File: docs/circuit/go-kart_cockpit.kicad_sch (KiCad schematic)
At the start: 37 parts, among them P1 Power, Q1 TIP120, SW1 SW_MEC_5E, X1 AVR-ISP-10, X10 Bluetooth-Modul, X11 Start/Stop/Rückwärts, X12 Taster rechts (male), X13 Taster links (male), X2 Display (male), X3 5V, X4 GND, X5 SDA, X6 24V Hupe, X7 J5, X8 J3, X9 SCL

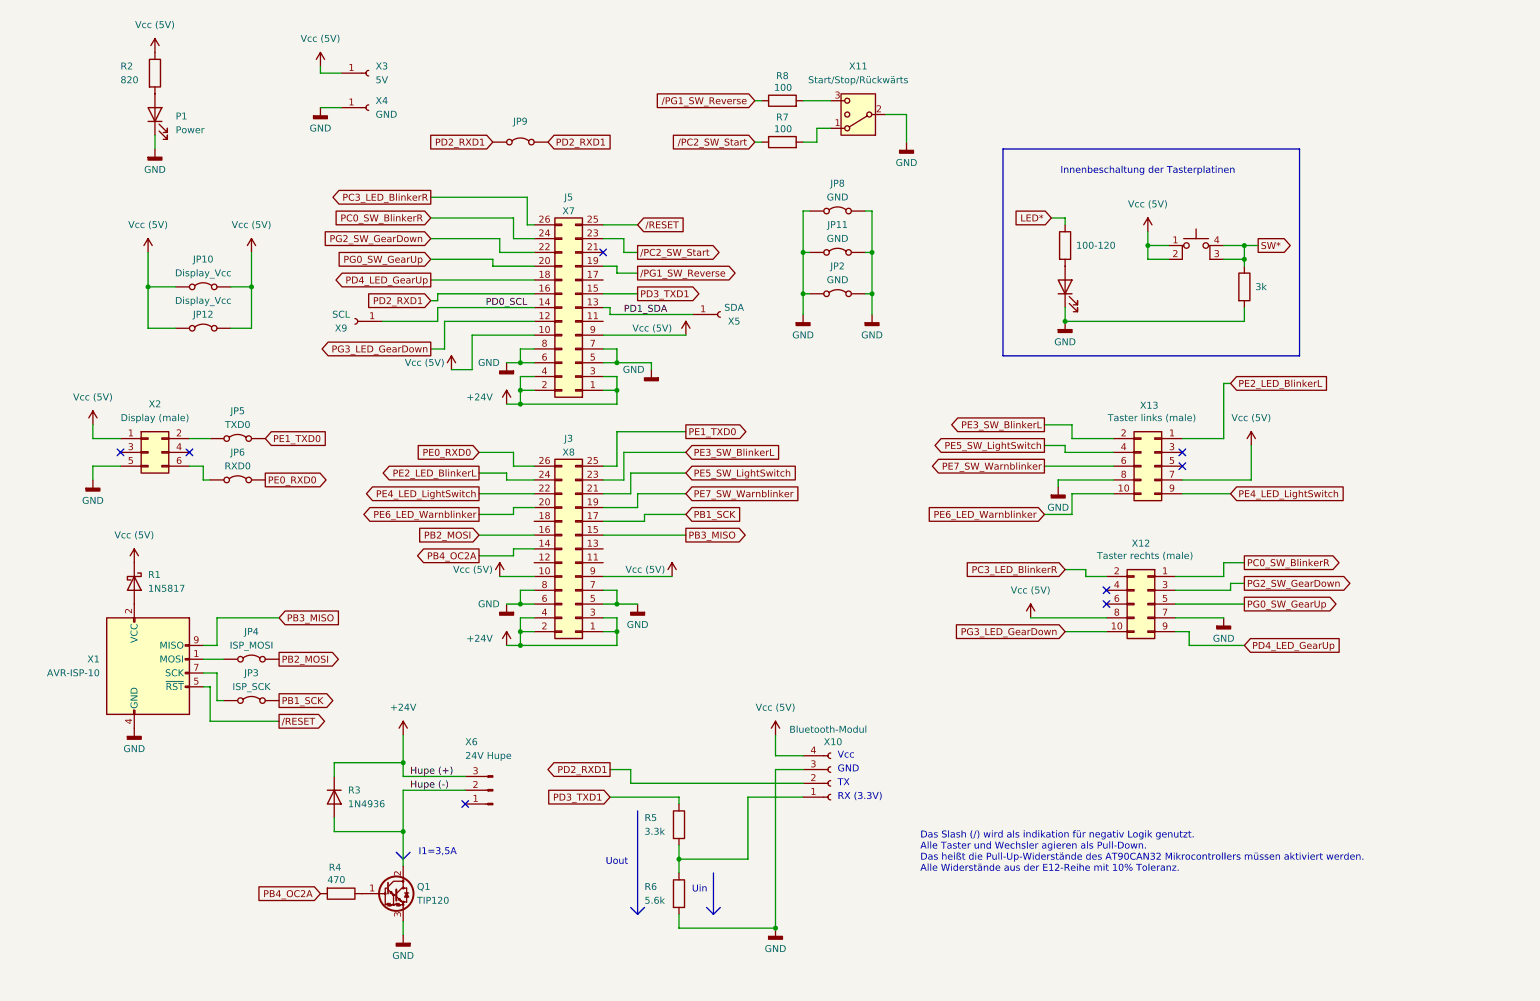
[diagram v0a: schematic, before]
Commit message: feat(circuit): final touches
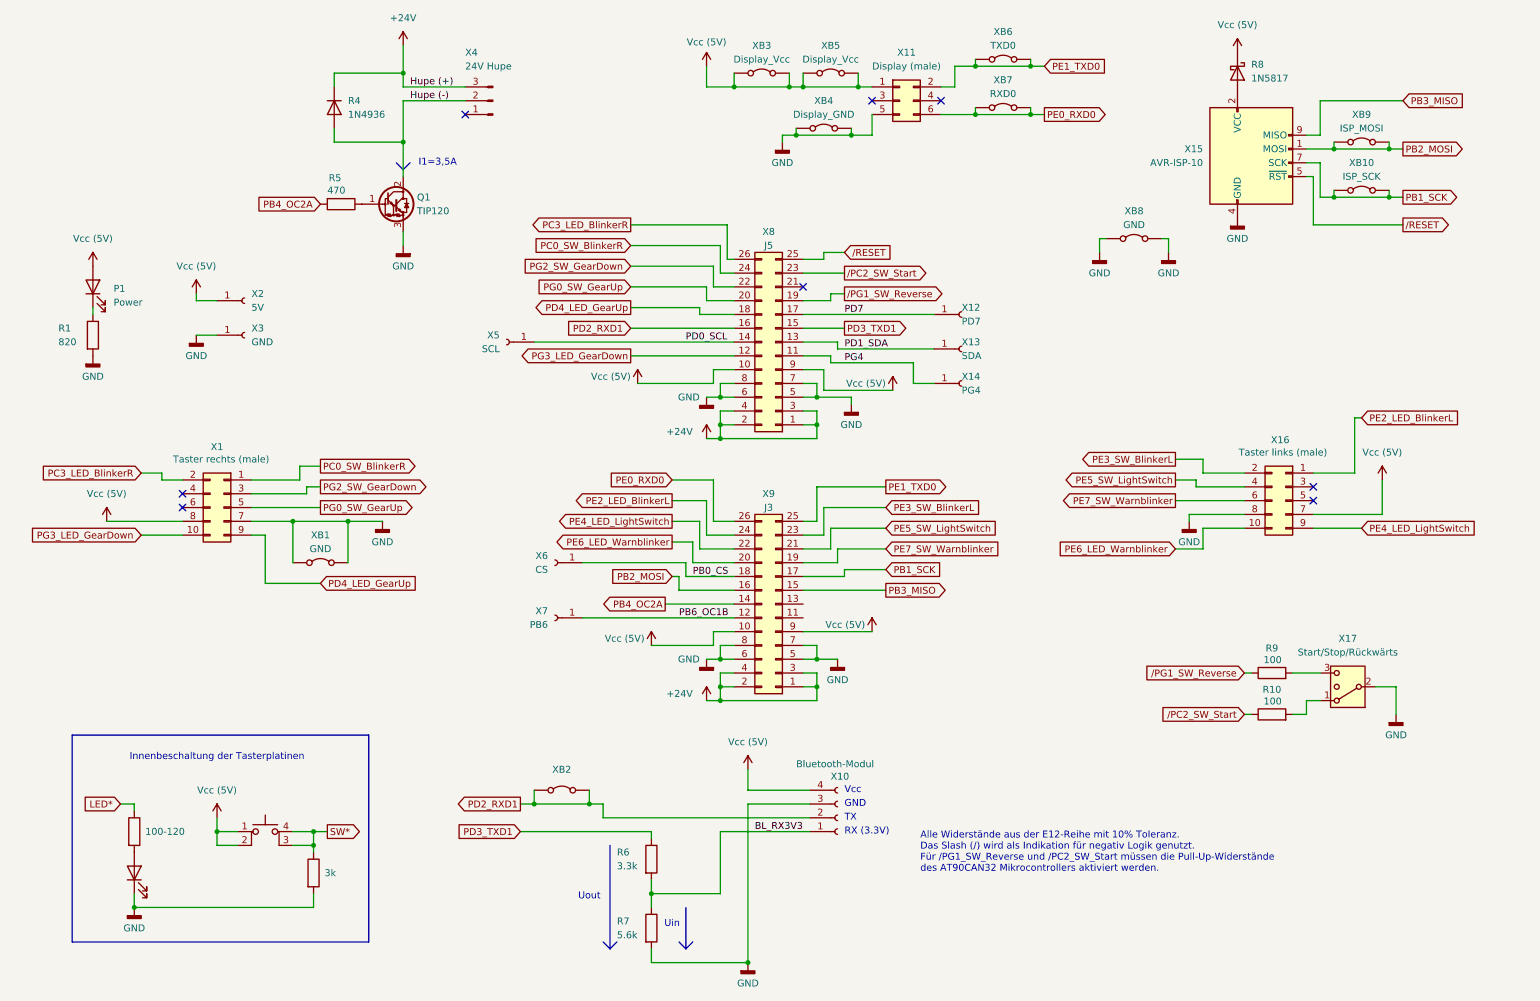
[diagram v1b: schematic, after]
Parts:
- removed JP10: Display_Vcc, Resistor_THT:R_Axial_DIN0207_L6.3mm_D2.5mm_P7.62mm_Horizontal, symbol Jumper:Jumper_2_Bridged
- removed JP12: Display_Vcc, Resistor_THT:R_Axial_DIN0207_L6.3mm_D2.5mm_P15.24mm_Horizontal, symbol Jumper:Jumper_2_Bridged
- removed JP3: ISP_SCK, Resistor_THT:R_Axial_DIN0207_L6.3mm_D2.5mm_P10.16mm_Horizontal, symbol Jumper:Jumper_2_Bridged
- removed JP4: ISP_MOSI, Resistor_THT:R_Axial_DIN0207_L6.3mm_D2.5mm_P15.24mm_Horizontal, symbol Jumper:Jumper_2_Bridged
- removed JP5: TXD0, Resistor_THT:R_Axial_DIN0207_L6.3mm_D2.5mm_P10.16mm_Horizontal, symbol Jumper:Jumper_2_Bridged
- removed JP6: RXD0, Resistor_THT:R_Axial_DIN0207_L6.3mm_D2.5mm_P10.16mm_Horizontal, symbol Jumper:Jumper_2_Bridged
- removed JP9: ~, Resistor_THT:R_Axial_DIN0207_L6.3mm_D2.5mm_P15.24mm_Horizontal, symbol Jumper:Jumper_2_Bridged
- added X12: PD7, Connector_PinSocket_2.54mm:PinSocket_1x01_P2.54mm_Vertical, symbol Connector:Conn_01x01_Socket
- added X14: PG4, Connector_PinSocket_2.54mm:PinSocket_1x01_P2.54mm_Vertical, symbol Connector:Conn_01x01_Socket
- added X6: CS, Connector_PinSocket_2.54mm:PinSocket_1x01_P2.54mm_Vertical, symbol Connector:Conn_01x01_Socket
- added X7: PB6, Connector_PinSocket_2.54mm:PinSocket_1x01_P2.54mm_Vertical, symbol Connector:Conn_01x01_Socket
- added XB10: ISP_SCK, Resistor_THT:R_Axial_DIN0207_L6.3mm_D2.5mm_P10.16mm_Horizontal, symbol Jumper:Jumper_2_Bridged
- added XB2: ~, Resistor_THT:R_Axial_DIN0207_L6.3mm_D2.5mm_P15.24mm_Horizontal, symbol Jumper:Jumper_2_Bridged
- added XB3: Display_Vcc, Resistor_THT:R_Axial_DIN0207_L6.3mm_D2.5mm_P7.62mm_Horizontal, symbol Jumper:Jumper_2_Bridged
- added XB5: Display_Vcc, Resistor_THT:R_Axial_DIN0207_L6.3mm_D2.5mm_P15.24mm_Horizontal, symbol Jumper:Jumper_2_Bridged
- added XB6: TXD0, Resistor_THT:R_Axial_DIN0207_L6.3mm_D2.5mm_P10.16mm_Horizontal, symbol Jumper:Jumper_2_Bridged
- added XB7: RXD0, Resistor_THT:R_Axial_DIN0207_L6.3mm_D2.5mm_P10.16mm_Horizontal, symbol Jumper:Jumper_2_Bridged
- added XB9: ISP_MOSI, Resistor_THT:R_Axial_DIN0207_L6.3mm_D2.5mm_P15.24mm_Horizontal, symbol Jumper:Jumper_2_Bridged
- XB4: renamed from JP8; value GND -> Display_GND
- renumbered R2 to R1, R7 to R10, R9 to R2, R10 to R3, R3 to R4, R4 to R5, R5 to R6, R6 to R7, R1 to R8, R8 to R9, X12 to X1, X2 to X11, X5 to X13, X1 to X15, X13 to X16, X11 to X17, X3 to X2, X4 to X3, X6 to X4, X9 to X5, X7 to X8, X8 to X9, JP11 to XB1, JP2 to XB8
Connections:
- net GND: now also R1.2; no longer P1.1 (K)
- net PB1_SCK: now also X15.7 (SCK), XB10.1 (A), XB10.2 (B)
- net PB2_MOSI: now also X15.1 (MOSI), XB9.1 (A), XB9.2 (B)
- net PD2_RXD1: now also XB2.1 (A), XB2.2 (B)
- net PE0_RXD0: now also X11.6 (Pin_6), XB7.1 (A), XB7.2 (B)
- net PE1_TXD0: now also X11.2 (Pin_2), XB6.1 (A), XB6.2 (B)
- net Vcc (5V): now also P1.2 (A), XB3.1 (A), XB3.2 (B), XB5.1 (A), XB5.2 (B); no longer R1.1
- net BL_RX3V3: now reaches R6.2, R7.1, X10.1 (Pin_1)
- net PG4: now reaches X8.11 (Pin_11)
- net PG4: now also X14.1 (Pin_1)
- net PD7: now reaches X8.17 (Pin_17)
- net PD7: now also X12.1 (Pin_1)
- net PB6_OC1B: now reaches X9.12 (Pin_12)
- net PB6_OC1B: now also X7.1 (Pin_1)
- net PB0_CS: now reaches X9.18 (Pin_18)
- net PB0_CS: now also X6.1 (Pin_1)
- new net: P1.1 (K), R1.1
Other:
- note added: "Alle Widerstände aus der E12-Reihe mit 10% Toleranz. Das Slash (/) wird als Indikation für negativ Logik genutzt. Für /PG1_SW_Reverse und /PC2_SW_Start müssen die Pull-Up-Widerstände des AT90CAN32 Mikrocontrollers aktiviert werden."
- note removed: "Das Slash (/) wird als indikation für negativ Logik genutzt. Alle Taster und Wechsler agieren als Pull-Down. Das heißt die Pull-Up-Widerstände des AT90CAN32 Mikrocontrollers müssen aktiviert werden. Alle Widerstände aus der E12-Reihe mit 10% Toleranz."
- title: go-kart_cockpit -> JCS-BK1091_GO-KART_Cockpitplatine
- moved on the sheet: P1, Q1, R1, R10, R4, R5, R6, R7, R8, R9, X1, X10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
